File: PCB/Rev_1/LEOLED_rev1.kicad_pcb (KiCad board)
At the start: 2 copper layers, 84.1 x 40 mm, 91 parts, among them J1 PHEONIX_MPT_1725698, J2 USB_MicroB, J3 PHOENIX_MPT_1725656, J4 WURTH_61300411121, J5 FTSH-105-01-F-DV-K, J7 PHOENIX_MPT_1725656, Q1 DMN65D8L-7, Q2 DMN65D8L-7, U1 BQ24210, U2 MAX1725, U3 TPS61169

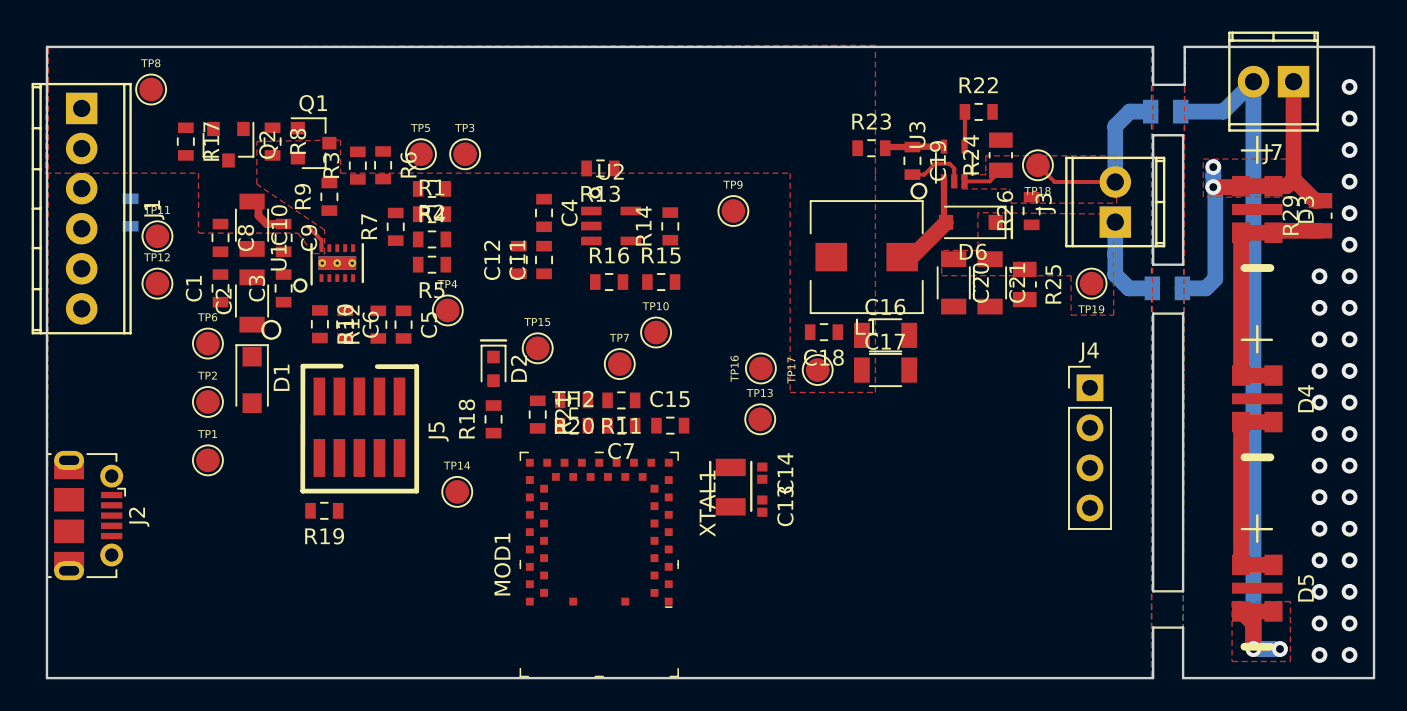
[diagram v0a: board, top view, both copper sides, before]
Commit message: layout editing
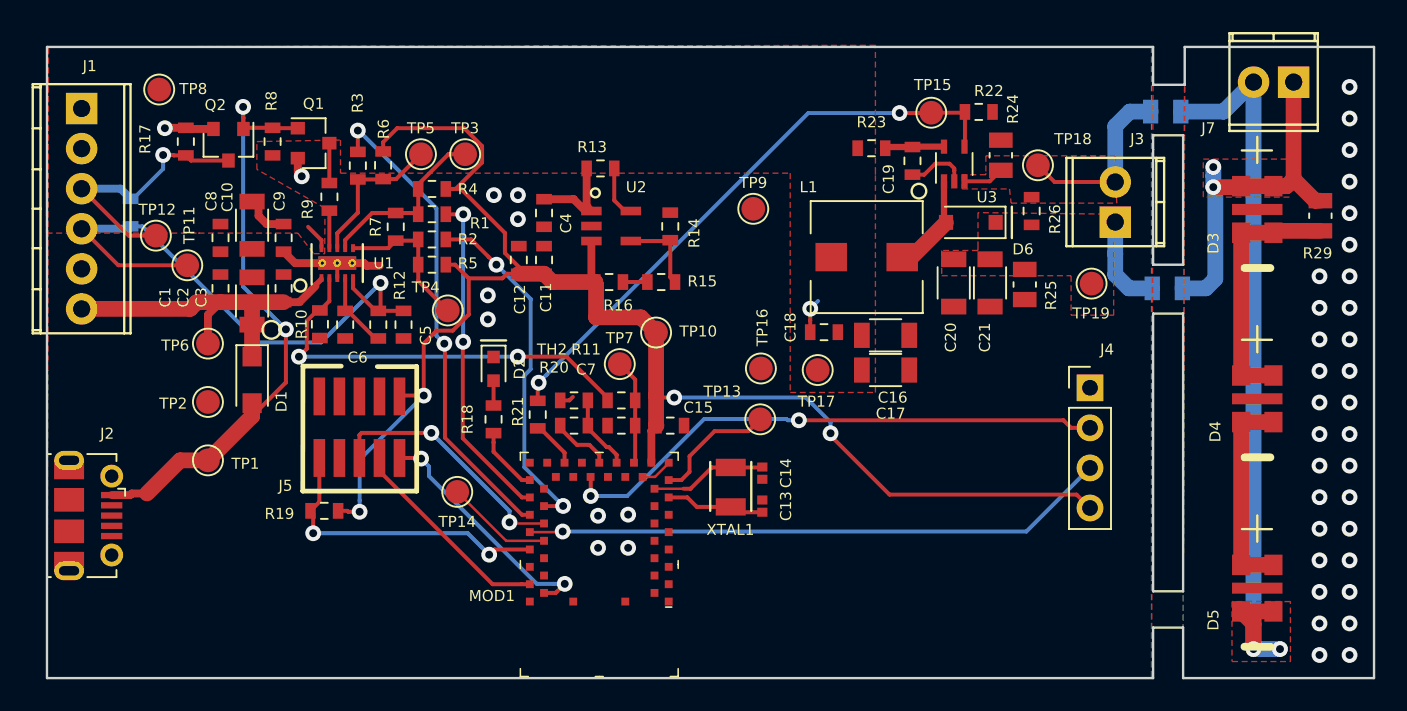
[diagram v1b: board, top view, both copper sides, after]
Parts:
- moved TP15 29.1 mm to (198.0, 102.2)
- moved TP12 3.04 mm to (148.9, 110.0)
- moved TP11 2.64 mm to (150.9, 111.8)
- moved TP9 1.27 mm to (186.8, 108.3)
- moved TP8 0.51 mm to (149.1, 100.7)
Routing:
- net VDD: track 0.00 -> 99.5 mm, vias 0 -> 4
- net /Power/VUSB: track 0.00 -> 42.3 mm, vias 0 -> 2
- net /Power/NTC_P: track 0.00 -> 37.5 mm, vias 0 -> 1
- net /BLE/UART_TX: track 0.00 -> 37.2 mm, vias 0 -> 1
- net Net-(R21-Pad1): track 2.21 -> 37.5 mm, vias 0 -> 2
- net /BLE/UART_RX: track 0.00 -> 35.1 mm, vias 0 -> 2
- net /Power/BQ_CHG: track 0.00 -> 30.5 mm, vias 0 -> 2
- net Net-(R10-Pad1): track 0.00 -> 26.8 mm, vias 0 -> 2
- net /Power/SOLAR_VDD: track 0.00 -> 23.1 mm
- net /Power/BQ_PG: track 0.00 -> 22.5 mm, vias 0 -> 2
- net /Power/BQ_EN: track 0.00 -> 21.1 mm, vias 0 -> 2
- net /BLE/RESET: track 0.00 -> 19.5 mm, vias 0 -> 2
- net /Power/NTC_N: track 0.00 -> 17.3 mm, vias 0 -> 1
- net /BLE/SWO: track 0.00 -> 16.0 mm, vias 0 -> 2
- net GND: track 3.88 -> 19.6 mm, vias 0 -> 12
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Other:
- net class Default: clearance 0.254 -> 0.2; trace_width 0.254 -> 0.16
- rule trace_clearance: 0.254 -> 0.2
- rule trace_min: 0.254 -> 0.16
